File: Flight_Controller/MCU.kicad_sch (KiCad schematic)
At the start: 1 part, among them U1 STM32H743VITx

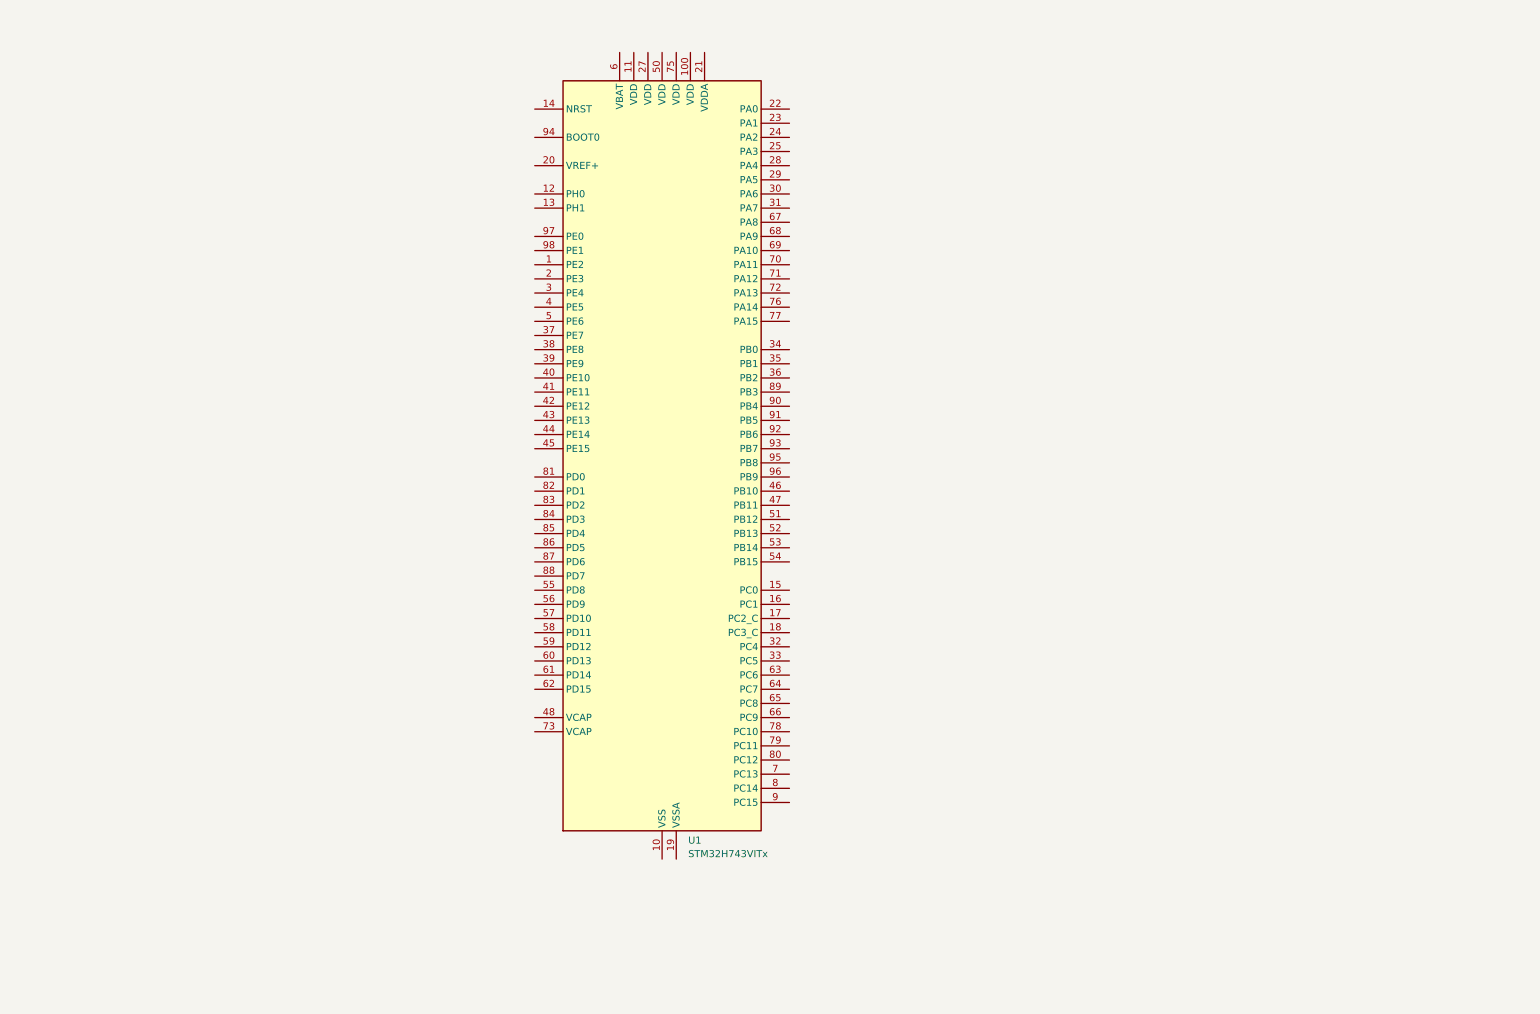
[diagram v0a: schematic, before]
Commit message: Schem V1 Done!
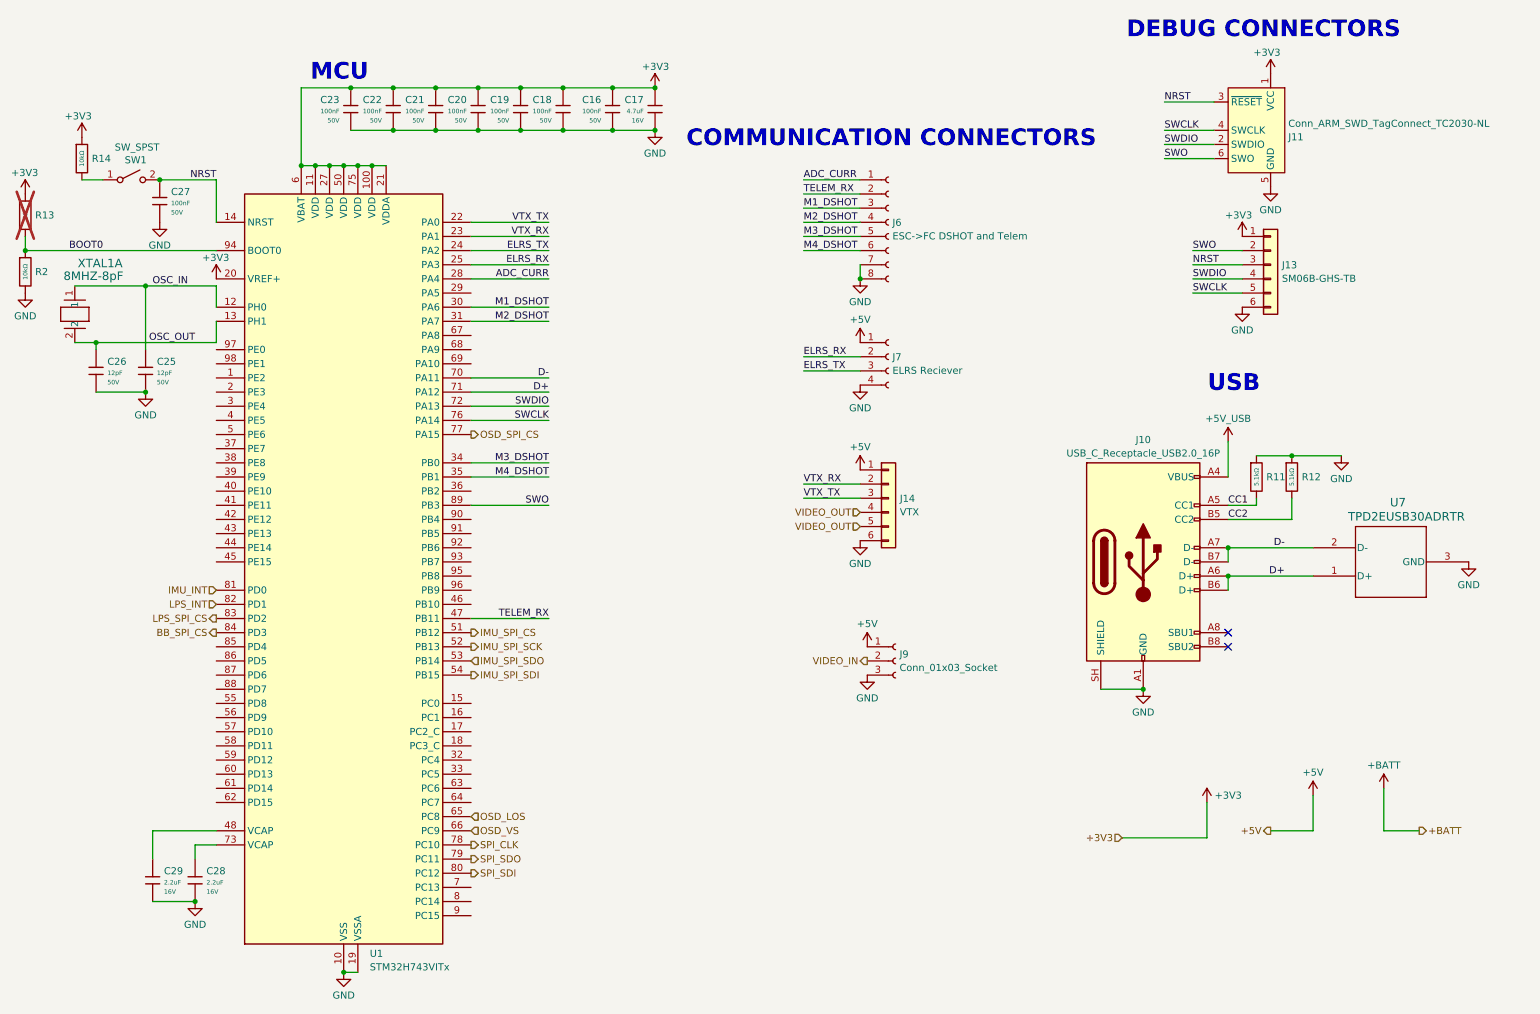
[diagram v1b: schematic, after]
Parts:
- added C16, C18, C19, C20, C21, C22, C23, C27: 100nF, PCM_JLCPCB:C_0603, symbol PCM_JLCPCB-Capacitors:0603,100nF
- added C17: 4.7uF, PCM_JLCPCB:C_0603, symbol PCM_JLCPCB-Capacitors:0603,4.7uF
- added C25, C26: 12pF, PCM_JLCPCB:C_0603, symbol PCM_JLCPCB-Capacitors:0603,12pF
- added C28, C29: 2.2uF, PCM_JLCPCB:C_0603, symbol PCM_JLCPCB-Capacitors:0603,2.2uF
- added J10: USB_C_Receptacle_USB2.0_16P, symbol Connector:USB_C_Receptacle_USB2.0_16P
- added J11: Conn_ARM_SWD_TagConnect_TC2030-NL, Connector:Tag-Connect_TC2030-IDC-NL_2x03_P1.27mm_Vertical, symbol Connector:Conn_ARM_SWD_TagConnect_TC2030-NL
- added J13: SM06B-GHS-TB, symbol Connector_Generic:Conn_01x06
- added J14: VTX, symbol Connector_Generic:Conn_01x06
- added J6: ESC->FC DSHOT and Telem, symbol Connector:Conn_01x08_Socket
- added J7: ELRS Reciever, symbol Connector:Conn_01x04_Socket
- added J9: Conn_01x03_Socket, symbol Connector:Conn_01x03_Socket
- added R11, R12: 5.1kΩ, PCM_JLCPCB:R_0603, symbol PCM_JLCPCB-Resistors:0603,5.1kΩ
- added R13: 0Ω, PCM_JLCPCB:R_0603, symbol PCM_JLCPCB-Resistors:0603,0Ω
- added R14, R2: 10kΩ, PCM_JLCPCB:R_0603, symbol PCM_JLCPCB-Resistors:0603,10kΩ
- added SW1: SW_SPST, symbol Switch:SW_SPST
- added U7: TPD2EUSB30ADRTR, Flight_Controller:DRT3-L, symbol Flight_Controller:TPD2EUSB30ADRTR
- added XTAL1: 8MHZ-8pF, Flight_Controller:XTAL_NX3225GD-8MHZ-STD-CRA-3_NDK-L, symbol Flight_Controller:NX3225GD-8MHZ-STD-CRA-3
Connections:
- net GND: now reaches U1.10 (VSS), U1.26 (VSS), U1.49 (VSS), U1.74 (VSS), U1.99 (VSS)
- net GND: now also U1.19 (VSSA), C16.2, C17.2, C18.2, C19.2, C20.2, C21.2, C22.2, C23.2, C25.1, C26.1, C27.1, C28.2, C29.2, J10.A1 (GND), J10.A12 (GND), J10.B1 (GND), J10.B12 (GND), J10.SH (SHIELD), J11.5 (GND), J13.6 (Pin_6), J14.6 (Pin_6), J6.7 (Pin_7), J6.8 (Pin_8), J7.4 (Pin_4), J9.3 (Pin_3), R11.1, R12.1, R2.2, U7.3 (GND)
- net +3V3: now reaches U1.100 (VDD)
- net +3V3: now also U1.11 (VDD), U1.20 (VREF+), U1.21 (VDDA), U1.27 (VDD), U1.50 (VDD), U1.6 (VBAT), U1.75 (VDD), C16.1, C17.1, C18.1, C19.1, C20.1, C21.1, C22.1, C23.1, J11.1 (VCC), J13.1 (Pin_1), R13.1, R14.1
- net OSC_IN: now reaches U1.12 (PH0)
- net OSC_IN: now also C25.2, XTAL1.1
- net OSC_OUT: now reaches U1.13 (PH1)
- net OSC_OUT: now also C26.2, XTAL1.2
- net NRST: now reaches U1.14 (NRST)
- net NRST: now also C27.2, J11.3 (~{RESET}), J13.3 (Pin_3), SW1.2 (B)
- net VTX_TX: now reaches U1.22 (PA0)
- net VTX_TX: now also J14.3 (Pin_3)
- net VTX_RX: now reaches U1.23 (PA1)
- net VTX_RX: now also J14.2 (Pin_2)
- net ELRS_TX: now reaches U1.24 (PA2)
- net ELRS_TX: now also J7.3 (Pin_3)
- net ELRS_RX: now reaches U1.25 (PA3)
- net ELRS_RX: now also J7.2 (Pin_2)
- net ADC_CURR: now reaches U1.28 (PA4)
- net ADC_CURR: now also J6.1 (Pin_1)
- net M1_DSHOT: now reaches U1.30 (PA6)
- net M1_DSHOT: now also J6.3 (Pin_3)
- net M2_DSHOT: now reaches U1.31 (PA7)
- net M2_DSHOT: now also J6.4 (Pin_4)
- net M3_DSHOT: now reaches U1.34 (PB0)
- net M3_DSHOT: now also J6.5 (Pin_5)
- net M4_DSHOT: now reaches U1.35 (PB1)
- net M4_DSHOT: now also J6.6 (Pin_6)
- net TELEM_RX: now reaches U1.47 (PB11)
- net TELEM_RX: now also J6.2 (Pin_2)
- net at U1.48 (VCAP): now also C29.1
- net IMU_SPI_CS: now reaches U1.51 (PB12)
- net IMU_SPI_SCK: now reaches U1.52 (PB13)
- net IMU_SPI_SDO: now reaches U1.53 (PB14)
- net IMU_SPI_SDI: now reaches U1.54 (PB15)
- net OSD_LOS: now reaches U1.65 (PC8)
- net OSD_VS: now reaches U1.66 (PC9)
- net D-: now reaches U1.70 (PA11)
- net D-: now also J10.A7 (D-), J10.B7 (D-), U7.2 (D-)
- net D+: now reaches U1.71 (PA12)
- net D+: now also J10.A6 (D+), J10.B6 (D+), U7.1 (D+)
- net SWDIO: now reaches U1.72 (PA13)
- net SWDIO: now also J11.2 (SWDIO), J13.4 (Pin_4)
- net at U1.73 (VCAP): now also C28.1
- net SWCLK: now reaches U1.76 (PA14)
- net SWCLK: now also J11.4 (SWCLK), J13.5 (Pin_5)
- net OSD_SPI_CS: now reaches U1.77 (PA15)
- net SPI_CLK: now reaches U1.78 (PC10)
- net SPI_SDO: now reaches U1.79 (PC11)
- net SPI_SDI: now reaches U1.80 (PC12)
- net IMU_INT: now reaches U1.81 (PD0)
- net LPS_INT: now reaches U1.82 (PD1)
- net LPS_SPI_CS: now reaches U1.83 (PD2)
- net BB_SPI_CS: now reaches U1.84 (PD3)
- net SWO: now reaches U1.89 (PB3)
- net SWO: now also J11.6 (SWO), J13.2 (Pin_2)
- net BOOT0: now reaches U1.94 (BOOT0)
- net BOOT0: now also R13.2, R2.1
- new net: R14.2, SW1.1 (A)
- new net +5V: J14.1 (Pin_1), J7.1 (Pin_1), J9.1 (Pin_1)
- new net +5V_USB: J10.A4 (VBUS), J10.A9 (VBUS), J10.B4 (VBUS), J10.B9 (VBUS)
- new net CC1: J10.A5 (CC1), R11.2
- new net CC2: J10.B5 (CC2), R12.2
- new net VIDEO_IN: J9.2 (Pin_2)
- new net VIDEO_OUT: J14.4 (Pin_4), J14.5 (Pin_5)
- no-connect marks 0 -> 2
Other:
- note added: "COMMUNICATION CONNECTORS"
- note added: "DEBUG CONNECTORS"
- note added: "MCU"
- note added: "USB"
- moved on the sheet: U1
